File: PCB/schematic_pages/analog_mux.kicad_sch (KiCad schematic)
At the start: 33 parts, among them U1 SS49E, U10 SS49E, U11 SS49E, U12 SS49E, U13 SS49E, U3 SS49E, U4 SS49E, U5 SS49E, U6 SS49E, U7 SS49E, U8 SS49E, U9 SS49E

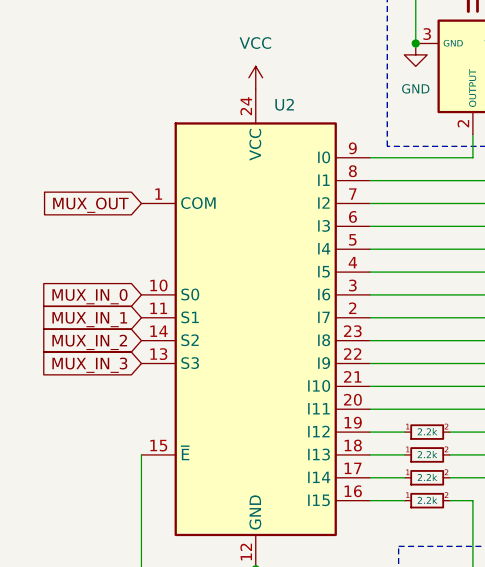
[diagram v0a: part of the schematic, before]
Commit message: repo rearrange
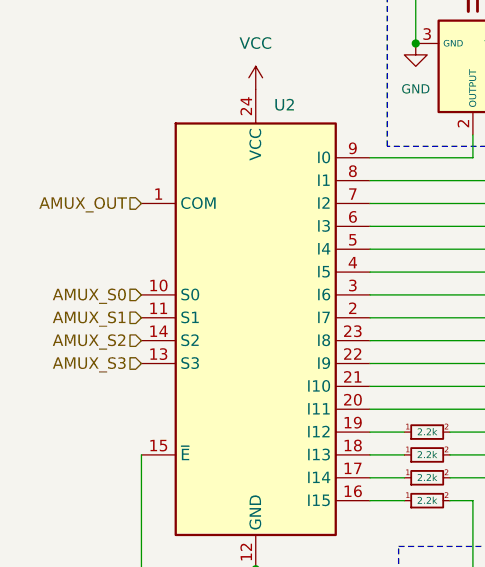
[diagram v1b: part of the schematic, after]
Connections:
- net MUX_IN_0 renamed AMUX_S0
- net MUX_IN_1 renamed AMUX_S1
- net MUX_IN_2 renamed AMUX_S2
- net MUX_IN_3 renamed AMUX_S3
- net MUX_OUT renamed AMUX_OUT
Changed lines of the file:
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@@
 		)
 	)
-	(global_label "MUX_IN_1"
+	(hierarchical_label "AMUX_OUT"
 		(shape input)
-		(at 25.4 102.87 180)
-		(fields_autoplaced yes)
+		(at 25.4 90.17 180)
 		(effects
 			(font
@@
 			(justify right)
 		)
-		(property "Intersheetrefs" "${INTERSHEET_REFS}"
-			(at 13.3434 102.87 0)
-			(effects
-				(font
-					(size 1.27 1.27)
-				)
-				(justify right)
-				(hide yes)
-			)
-		)
 	)
-	(global_label "MUX_OUT"
+	(hierarchical_label "AMUX_S1"
 		(shape input)
-		(at 25.4 90.17 180)
-		(fields_autoplaced yes)
+		(at 25.4 102.87 180)
 		(effects
 			(font
@@
 			(justify right)
 		)
-		(property "Intersheetrefs" "${INTERSHEET_REFS}"
-			(at 13.8272 90.17 0)
-			(effects
-				(font
-					(size 1.27 1.27)
-				)
-				(justify right)
-				(hide yes)
-			)
-		)
 	)
-	(global_label "MUX_IN_0"
+	(hierarchical_label "AMUX_S0"
 		(shape input)
 		(at 25.4 100.33 180)
-		(fields_autoplaced yes)
 		(effects
 			(font
@@
 			(justify right)
 		)
-		(property "Intersheetrefs" "${INTERSHEET_REFS}"
-			(at 13.3434 100.33 0)
-			(effects
-				(font
-					(size 1.27 1.27)
-				)
-				(justify right)
-				(hide yes)
-			)
-		)
 	)
-	(global_label "MUX_IN_3"
+	(hierarchical_label "AMUX_S2"
 		(shape input)
-		(at 25.4 107.95 180)
-		(fields_autoplaced yes)
+		(at 25.4 105.41 180)
 		(effects
 			(font
@@
 			(justify right)
 		)
-		(property "Intersheetrefs" "${INTERSHEET_REFS}"
-			(at 13.3434 107.95 0)
-			(effects
-				(font
-					(size 1.27 1.27)
-				)
-				(justify right)
-				(hide yes)
-			)
-		)
 	)
-	(global_label "MUX_IN_2"
+	(hierarchical_label "AMUX_S3"
 		(shape input)
-		(at 25.4 105.41 180)
-		(fields_autoplaced yes)
+		(at 25.4 107.95 180)
 		(effects
 			(font
@@
 			(justify right)
 		)
-		(property "Intersheetrefs" "${INTERSHEET_REFS}"
-			(at 13.3434 105.41 0)
-			(effects
-				(font
-					(size 1.27 1.27)
-				)
-				(justify right)
-				(hide yes)
-			)
-		)
 	)
